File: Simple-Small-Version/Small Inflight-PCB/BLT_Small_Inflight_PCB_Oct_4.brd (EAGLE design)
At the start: 65.6 x 58.4 mm, 8 parts

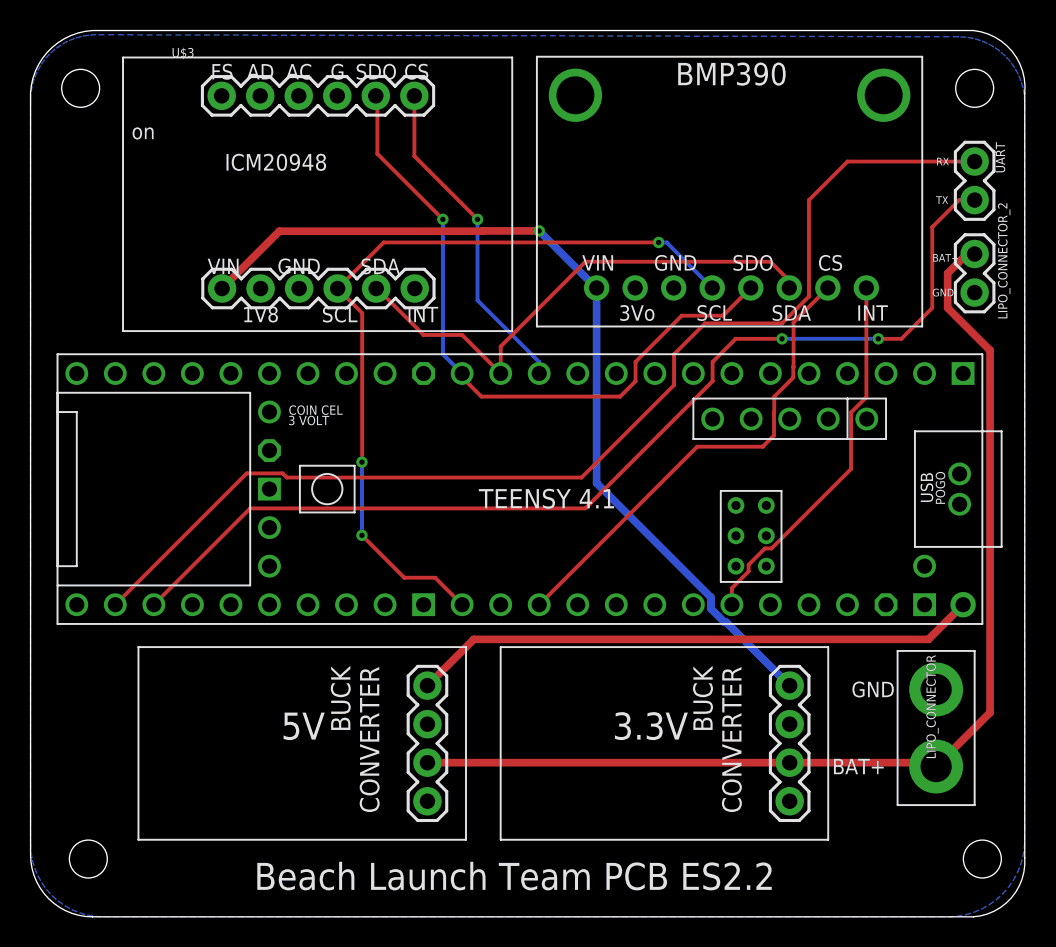
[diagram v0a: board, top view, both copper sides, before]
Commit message: Updated files
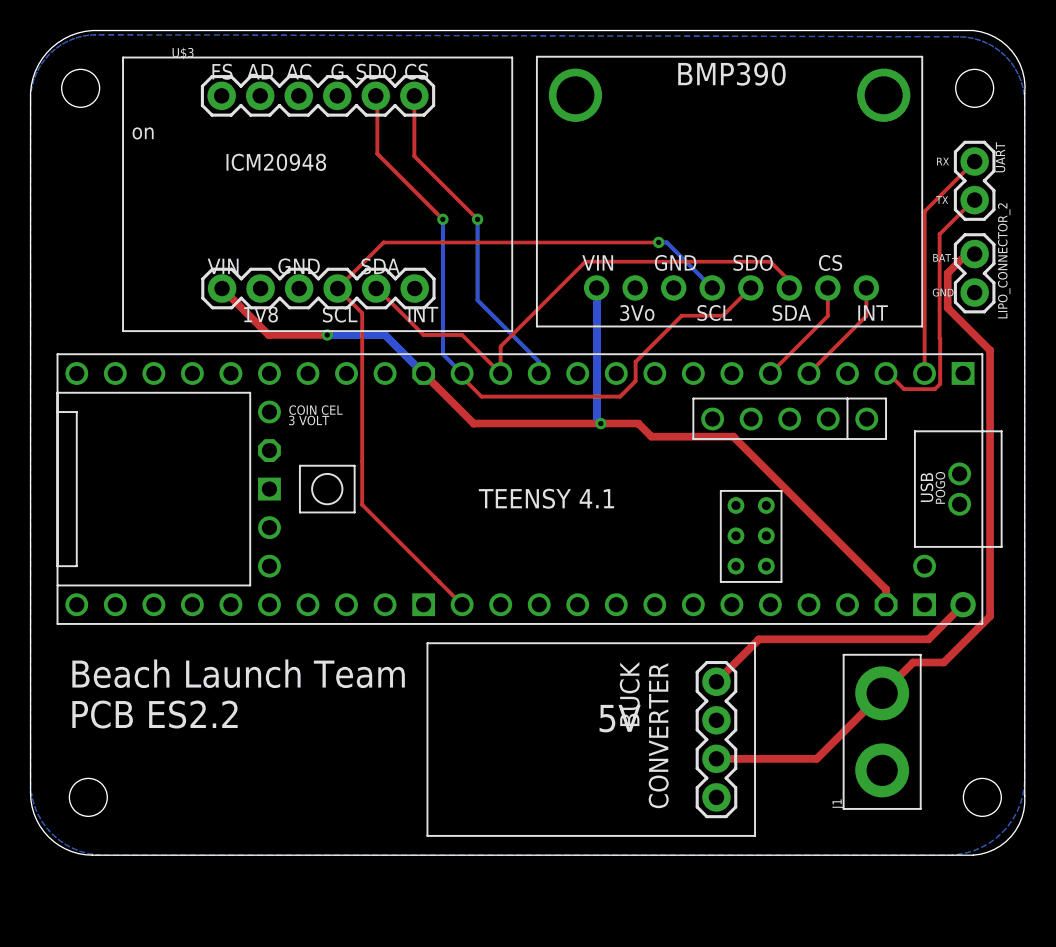
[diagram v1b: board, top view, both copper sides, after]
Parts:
- removed LIPO_CONNECTOR: (no value), SparkFun-Connectors:1X02_XTRA_BIG
- removed U$4: BUCK_CONVERTER3.3V, BLTFootprints:1X04
- added J1: (no value), SparkFun-Connectors:1X02_XTRA_BIG
- moved U$6 19.1 mm to (60.2, 52.1)
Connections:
- net 3.3V: now also U$1.3V3-1, U$1.3V3-3; no longer U$4.VO+
- net BAT+: now also J1.2; no longer LIPO_CONNECTOR.2, U$4.IN+
- net BMPINT: now also U$1.3-LRCLK2; no longer U$1.20-A6/TX5/LRCLK1
- net CS2: now also U$1.4-BCLK2; no longer U$1.15-A1/RX3/SPDIF_IN
- net GND: now also J1.1; no longer LIPO_CONNECTOR.1, U$4.GND
- net RX: now also U$1.0-RX1/CS1/CRX2; no longer U$1.34-RX8
- net TX: now also U$1.1-TX1/MISO1/CTX2; no longer U$1.35-TX8
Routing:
- net RX: track 73.9 -> 15.3 mm
- net TX: track 69.0 -> 17.3 mm, vias 2 -> 0
- net CS2: track 31.3 -> 7.21 mm
- net BAT+: track 71.6 -> 48.0 mm
- net 5V: track 37.5 -> 18.4 mm
- net BMPINT: track 24.8 -> 7.21 mm
- net 3.3V: track 59.4 -> 62.0 mm, vias 1 -> 2
- net SCK: track 52.6 -> 51.4 mm, vias 3 -> 1
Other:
- board size 65.6 x 58.4 mm -> 65.6 x 54.4 mm
- board text removed: "3.3V"
